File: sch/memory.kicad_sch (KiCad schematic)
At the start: 6 parts

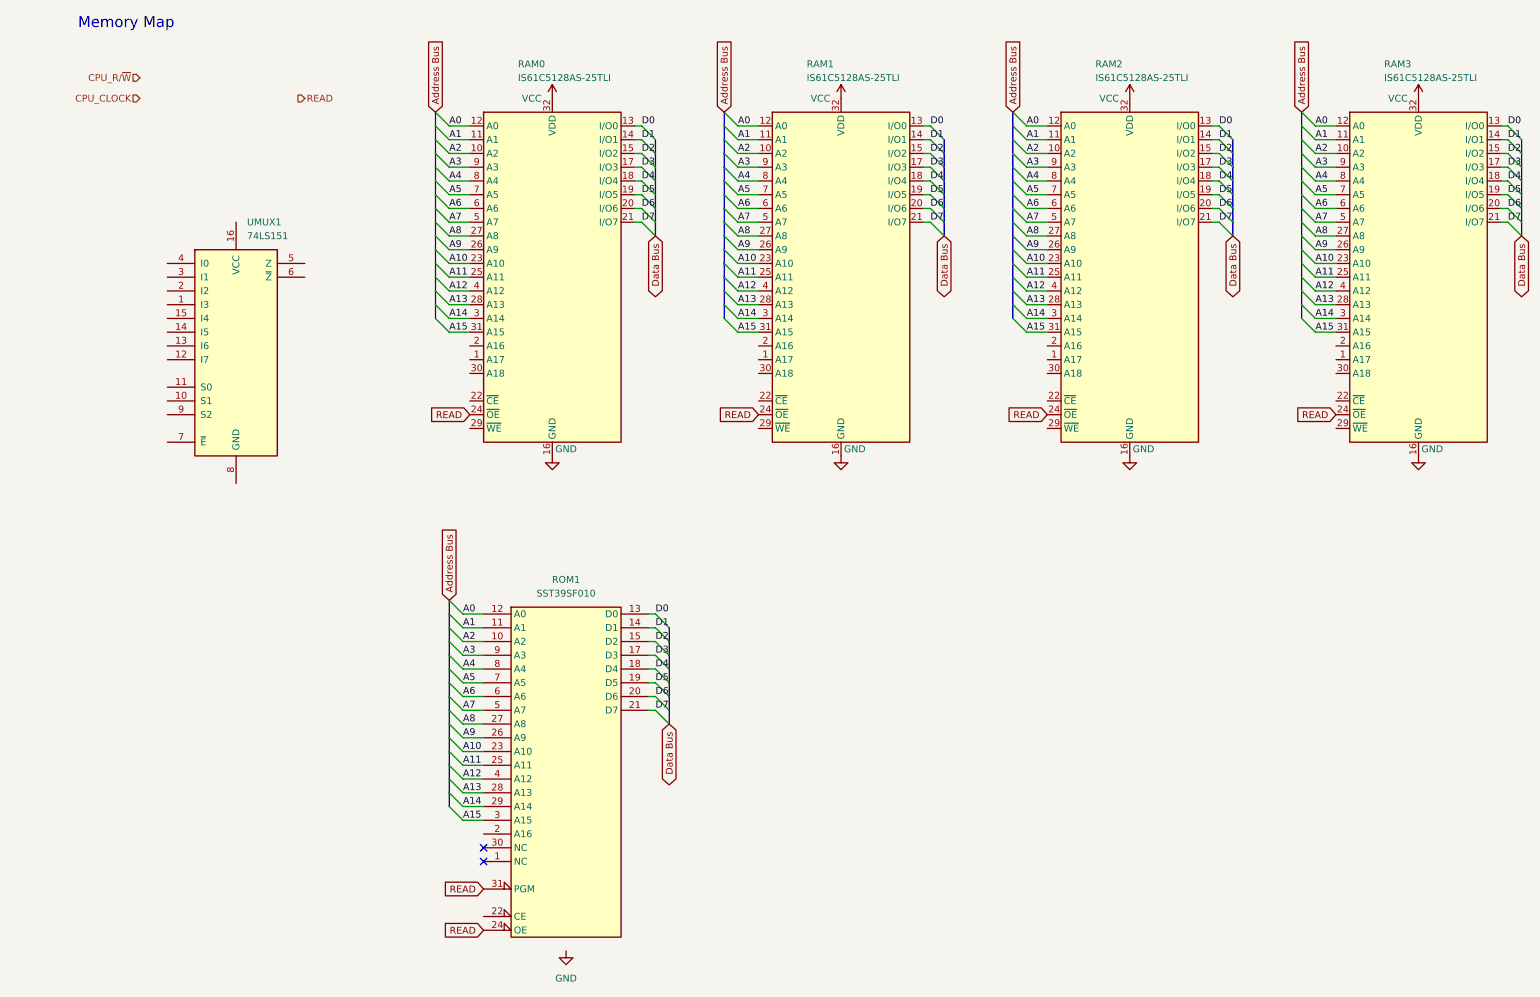
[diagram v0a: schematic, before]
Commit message: Memory Module
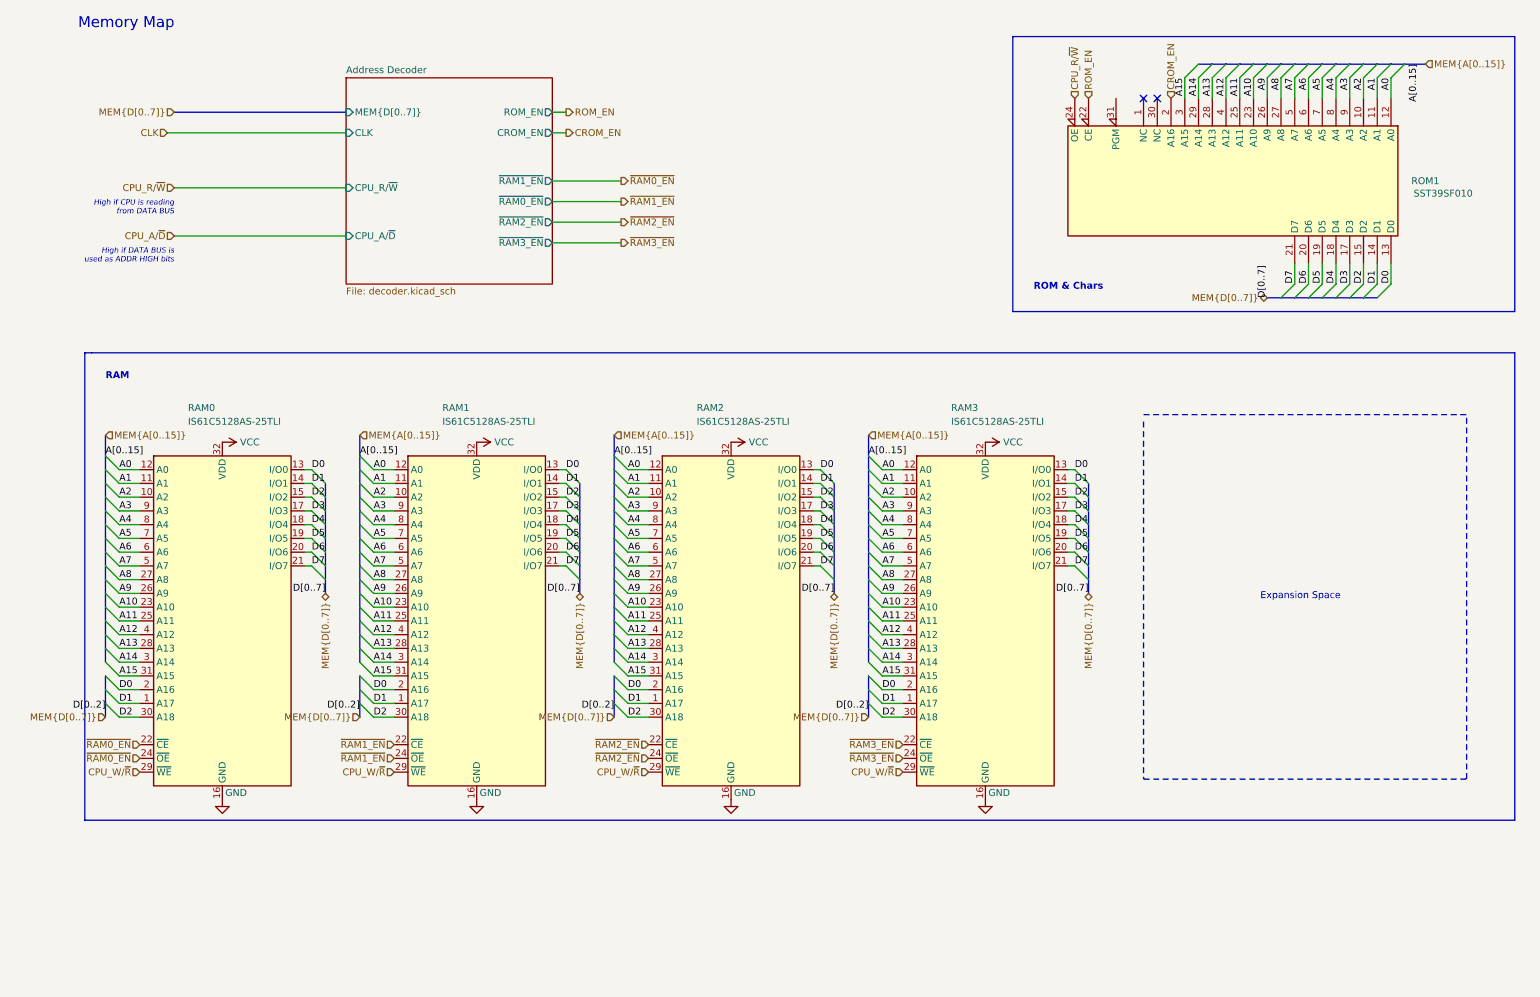
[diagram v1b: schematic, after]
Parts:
- removed UMUX1: 74LS151, Package_DIP:DIP-18_W7.62mm_SMDSocket_SmallPads, symbol 74xx:74LS151
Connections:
- net CPU_R/~{W}: now also ROM1.24 (OE)
- net D0: now also RAM0.2 (A16), RAM1.2 (A16), RAM2.2 (A16), RAM3.2 (A16)
- net D1: now also RAM0.1 (A17), RAM1.1 (A17), RAM2.1 (A17), RAM3.1 (A17)
- net D2: now also RAM0.30 (A18), RAM1.30 (A18), RAM2.30 (A18), RAM3.30 (A18)
- net ~{RAM2_EN}: now reaches RAM2.22 (~{CE})
- net ~{RAM2_EN}: now also RAM2.24 (~{OE})
- net CPU_W/~{R}: now reaches RAM2.29 (~{WE})
- net CPU_W/~{R}: now also RAM0.29 (~{WE}), RAM1.29 (~{WE}), RAM3.29 (~{WE})
- net ~{RAM1_EN}: now reaches RAM1.22 (~{CE})
- net ~{RAM1_EN}: now also RAM1.24 (~{OE})
- net ~{RAM0_EN}: now reaches RAM0.22 (~{CE})
- net ~{RAM0_EN}: now also RAM0.24 (~{OE})
- net ~{RAM3_EN}: now reaches RAM3.22 (~{CE})
- net ~{RAM3_EN}: now also RAM3.24 (~{OE})
- net CROM_EN: now reaches ROM1.2 (A16)
- net ROM_EN: now reaches ROM1.22 (CE)
- removed net READ: RAM0.24 (~{OE}), RAM1.24 (~{OE}), RAM2.24 (~{OE}), RAM3.24 (~{OE}), ROM1.24 (OE), ROM1.31 (PGM)
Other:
- added sheet Address Decoder (decoder.kicad_sch)
- note added: "Expansion Space"
- note added: "High if CPU is reading from DATA BUS"
- note added: "High if DATA BUS is used as ADDR HIGH bits"
- note added: "RAM"
- note added: "ROM & Chars"
- moved on the sheet: RAM0, RAM1, RAM2, RAM3, ROM1
